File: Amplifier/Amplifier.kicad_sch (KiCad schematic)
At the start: 28 parts, among them J1 Conn_01x01_Pin, J10 Conn_01x01_Pin, J11 Conn_01x01_Pin, J2 Conn_01x01_Pin, J9 Conn_01x10, Q1 JFE2140D, Q2 Q_NJFET_DSG, U16 LTC6268xS8, U2 LMP7721

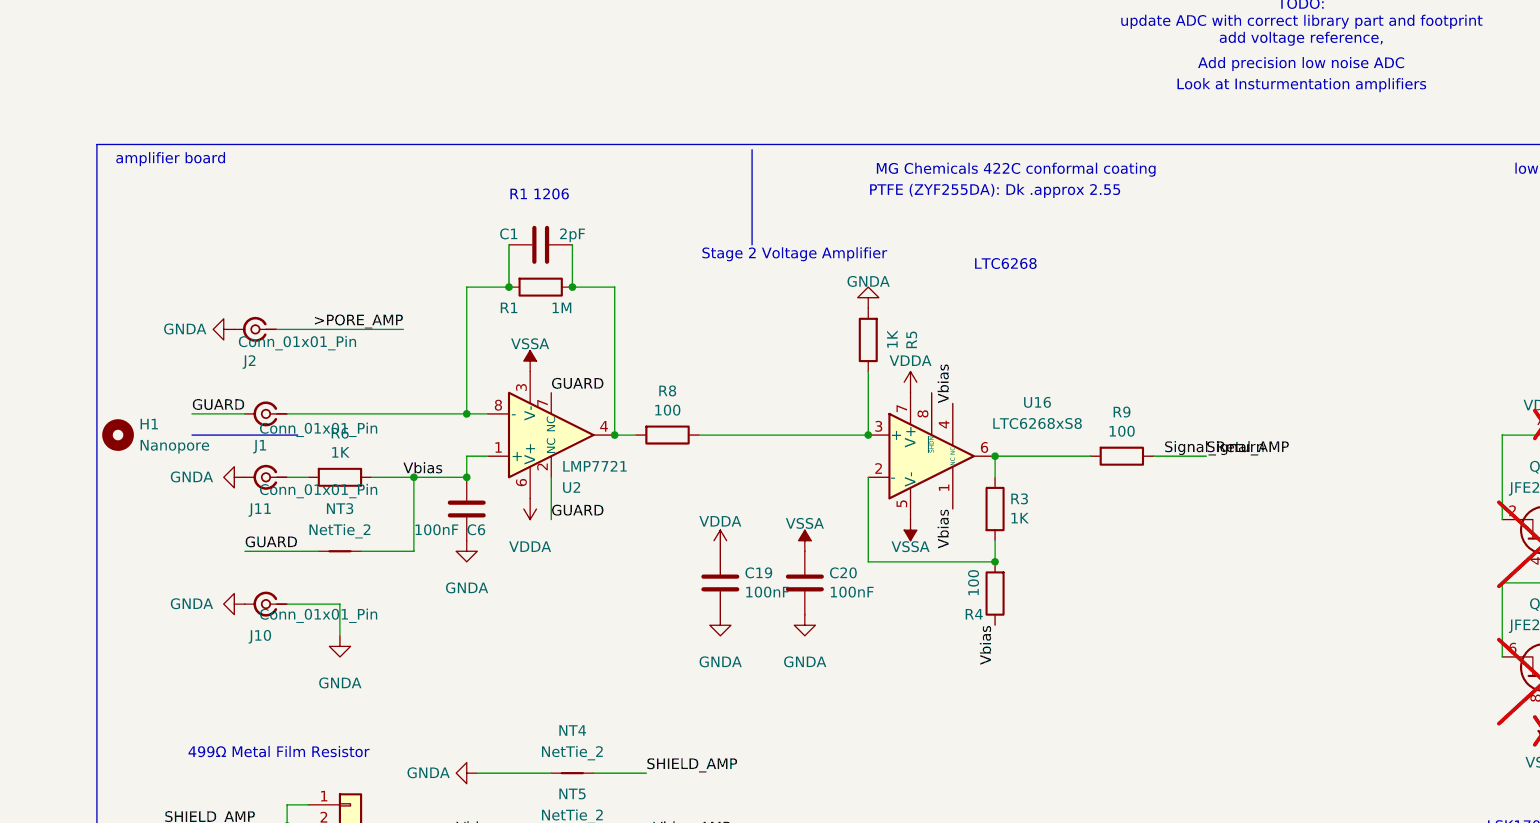
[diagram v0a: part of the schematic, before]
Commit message: Signed-off-by: lokimetasmith <lokimail@gmail.com>
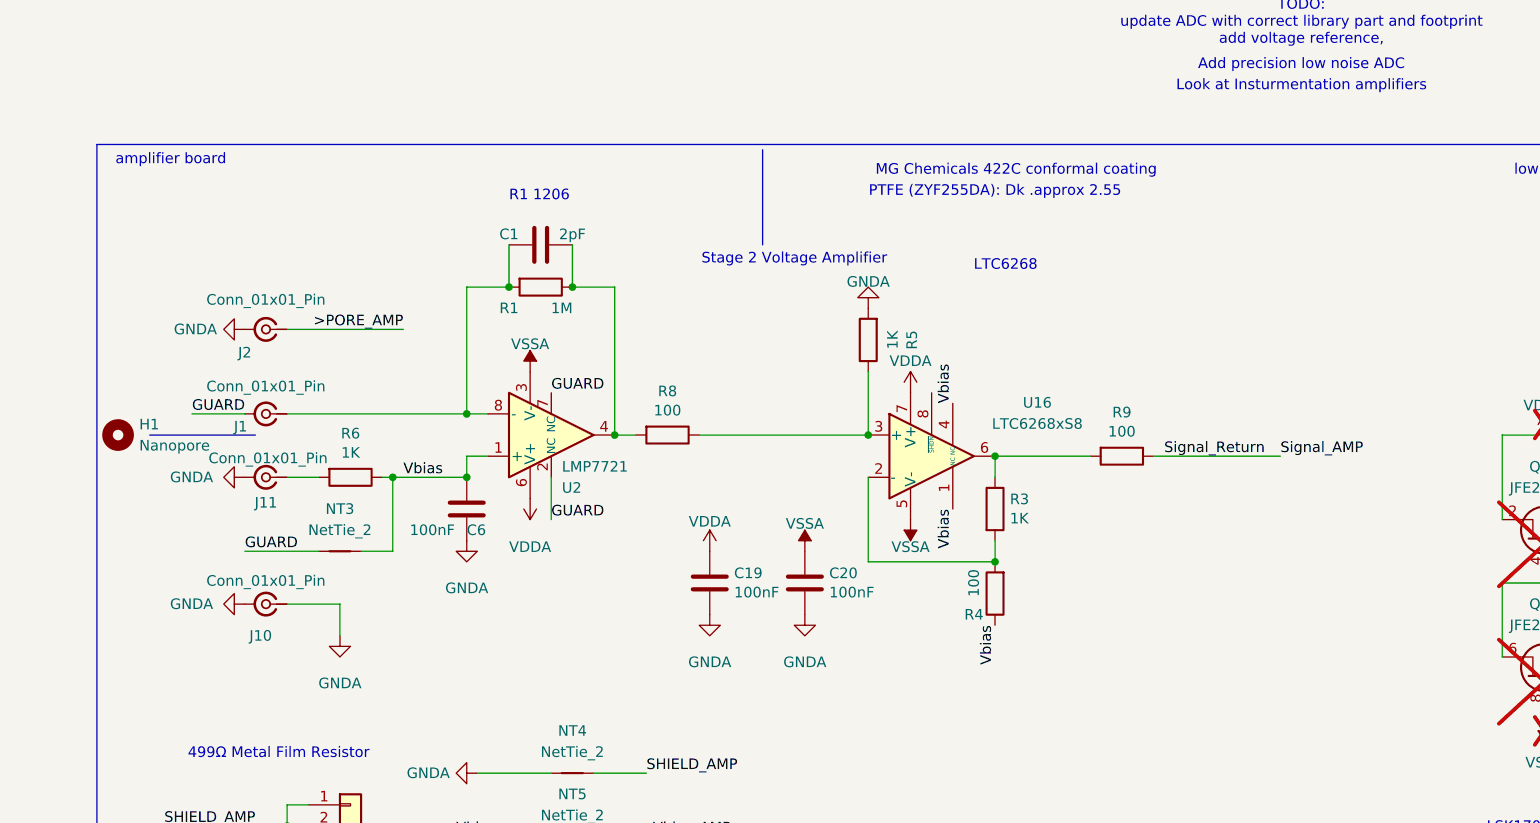
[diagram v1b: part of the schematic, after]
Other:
- moved on the sheet: C19, J2, R6

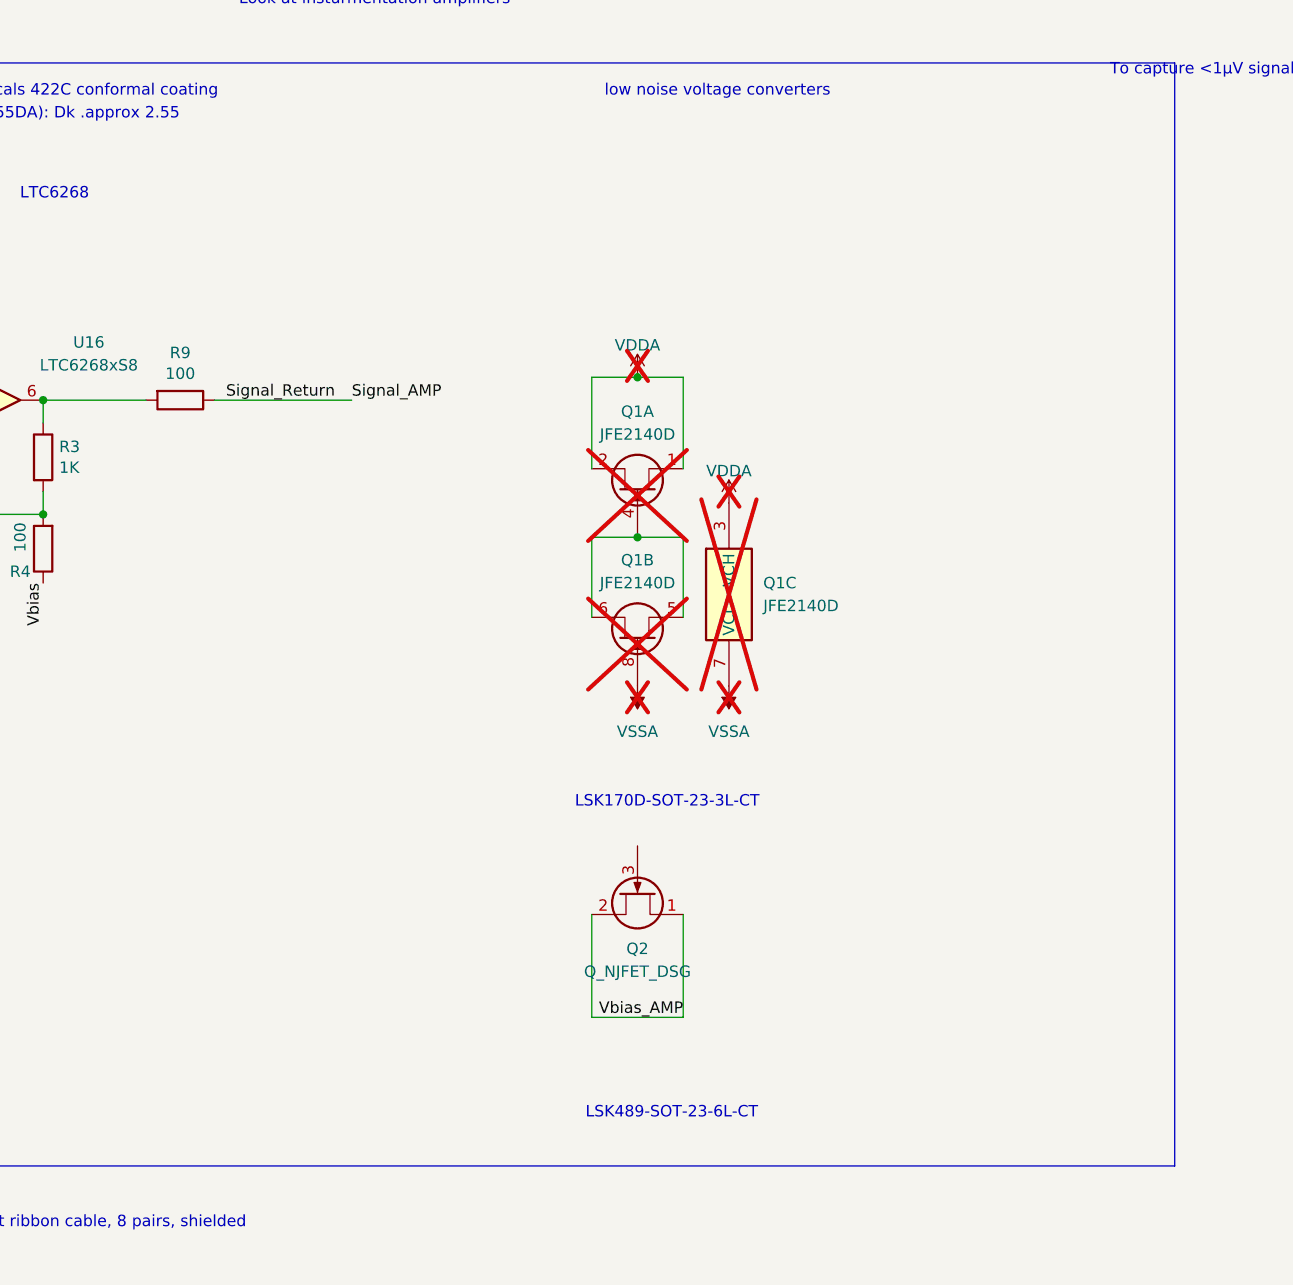
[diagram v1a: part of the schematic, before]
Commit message: Signed-off-by: lokimetasmith <lokimail@gmail.com>
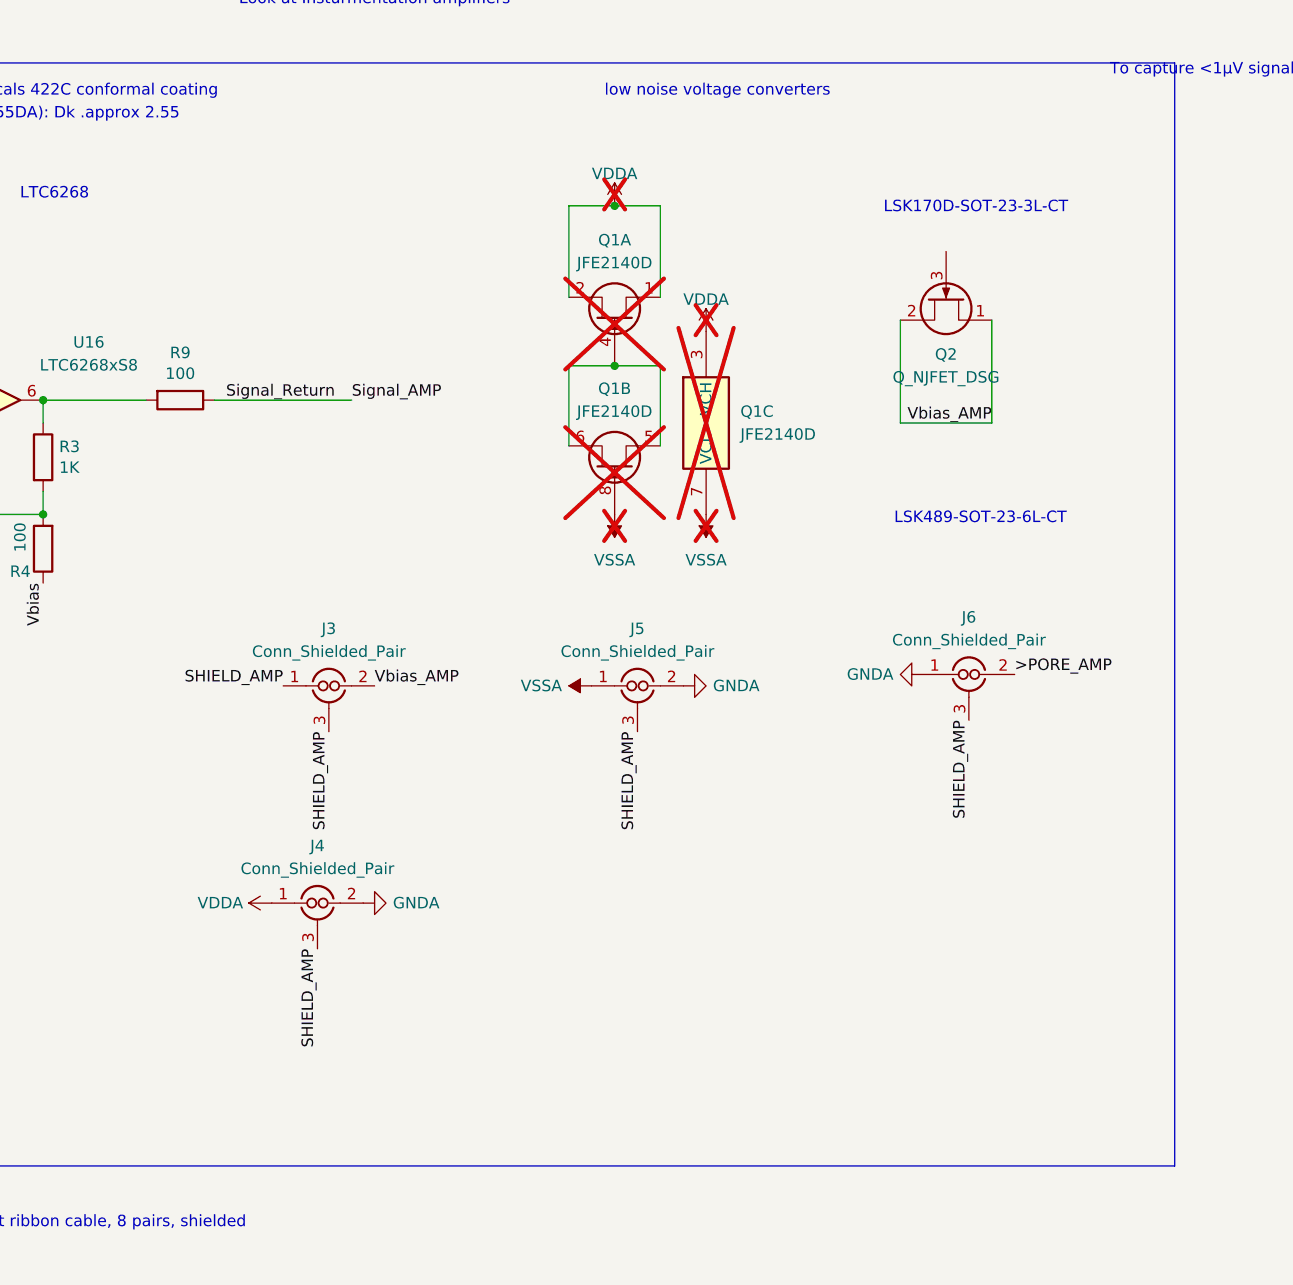
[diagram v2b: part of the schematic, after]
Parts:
- added J3, J4, J5, J6: Conn_Shielded_Pair, symbol Connector:Conn_Shielded_Pair
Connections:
- net >PORE_AMP: now also J6.2 (In2)
- net GNDA: now also J4.2 (In2), J5.2 (In2), J6.1 (In1)
- net SHIELD_AMP: now also J3.1 (In1), J3.3 (Ext), J4.3 (Ext), J5.3 (Ext), J6.3 (Ext)
- net VDDA: now also J4.1 (In1)
- net VSSA: now also J5.1 (In1)
- net Vbias_AMP: now also J3.2 (In2)
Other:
- moved on the sheet: Q1A, Q1B, Q1C, Q2
